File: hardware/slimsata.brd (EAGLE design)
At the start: 100 x 80 mm, 2 parts

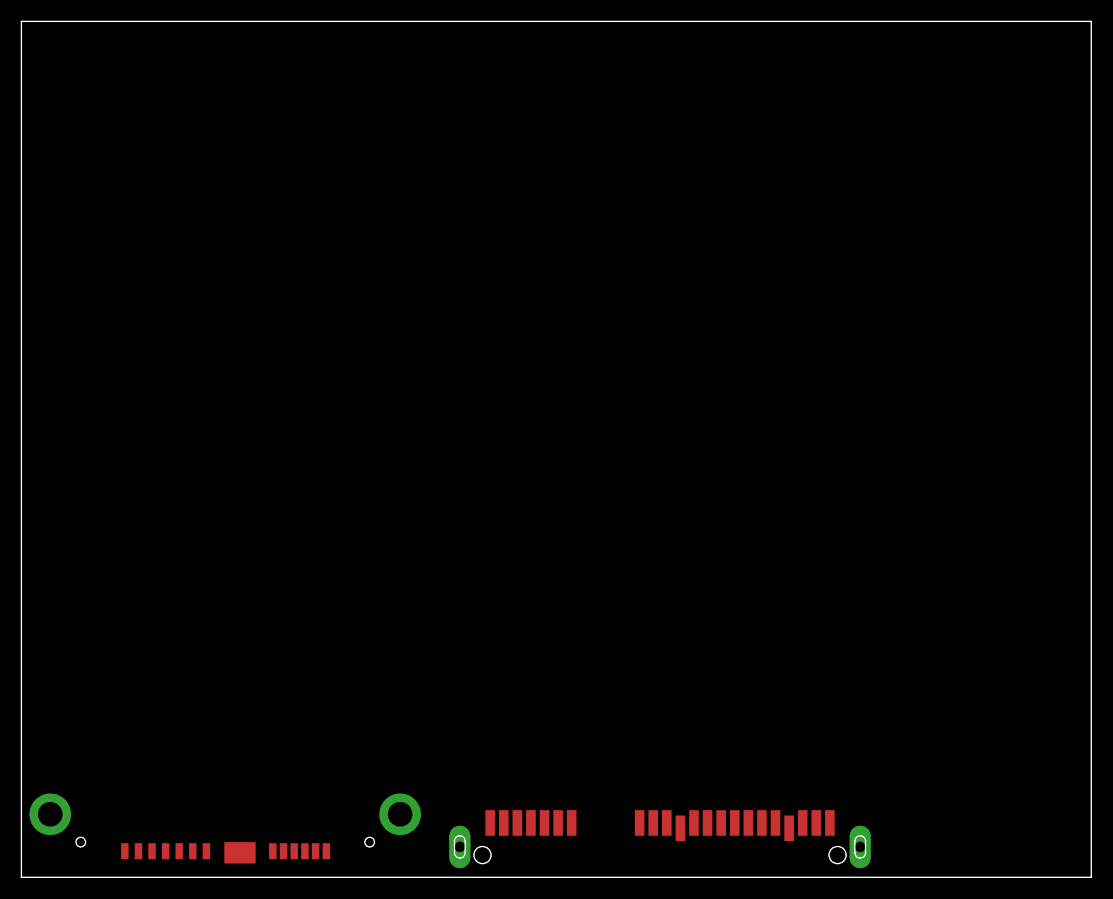
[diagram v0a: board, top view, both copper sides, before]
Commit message: Stecker neu platziert
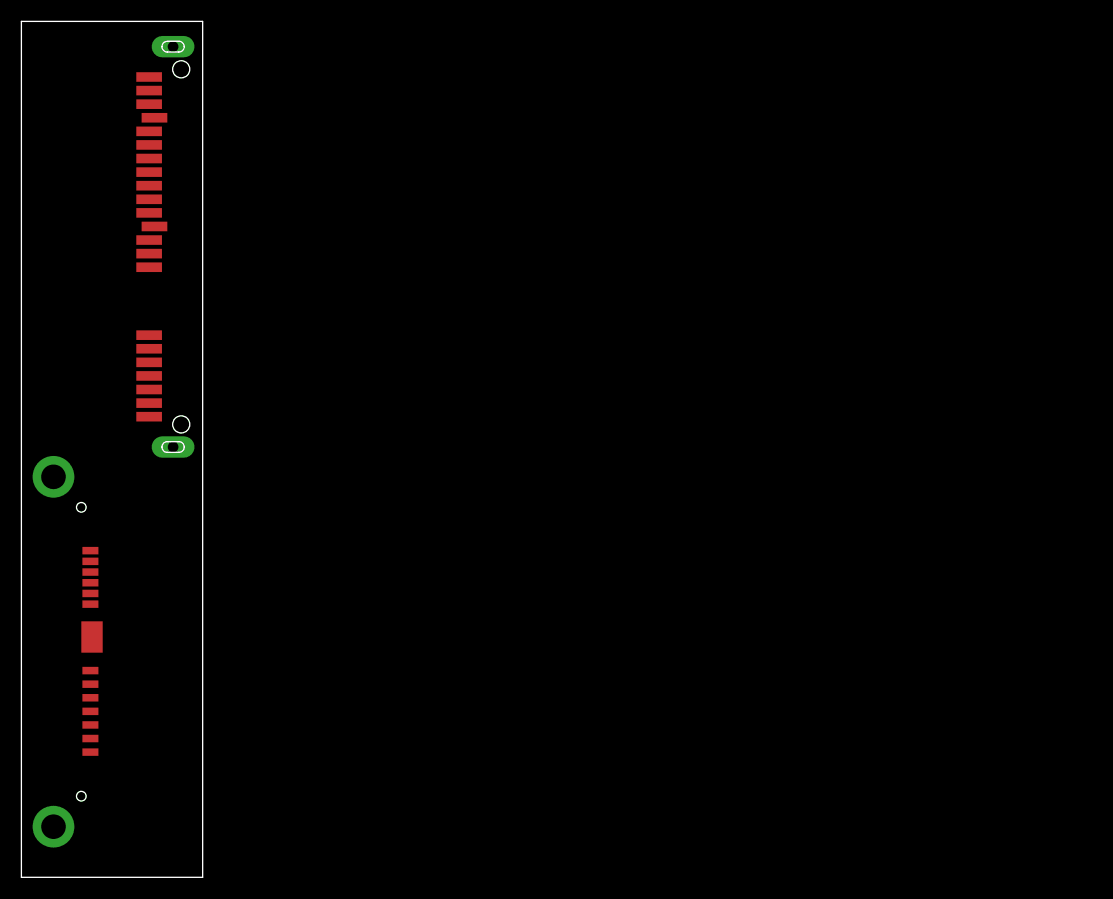
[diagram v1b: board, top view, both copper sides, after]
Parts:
- moved CON1 72.8 mm to (17.0, 58.9), turned to 90 degrees
- moved CON2 22.6 mm to (0.00, 21.1), turned to 270 degrees
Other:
- board size 100 x 80 mm -> 16.9 x 80 mm
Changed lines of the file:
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@@
 <board>
 <plain>
-<wire x1="0" y1="0" x2="100" y2="0" width="0" layer="20"/>
-<wire x1="100" y1="0" x2="100" y2="80" width="0" layer="20"/>
-<wire x1="100" y1="80" x2="0" y2="80" width="0" layer="20"/>
+<wire x1="0" y1="0" x2="16.942" y2="0" width="0" layer="20"/>
+<wire x1="16.942" y1="0" x2="16.942" y2="80" width="0" layer="20"/>
+<wire x1="16.942" y1="80" x2="0" y2="80" width="0" layer="20"/>
 <wire x1="0" y1="80" x2="0" y2="0" width="0" layer="20"/>
 </plain>
@@
 </autorouter>
 <elements>
-<element name="CON1" library="sata" package="MOLEX_47018" value="" x="59.69" y="0"/>
-<element name="CON2" library="sata" package="MOLEX_47300-1005" value="" x="19.05" y="8.89" rot="R180"/>
+<element name="CON1" library="sata" package="MOLEX_47018" value="" x="17.018" y="58.928" rot="R90"/>
+<element name="CON2" library="sata" package="MOLEX_47300-1005" value="" x="0" y="21.082" rot="R270"/>
 </elements>
 <signals>
@@
 <contactref element="CON2" pad="P6"/>
 <contactref element="CON2" pad="P5"/>
-<wire x1="35.4" y1="5.89" x2="40.98" y2="2.84" width="0" layer="19" extent="1-1"/>
-<wire x1="28.5" y1="2.44" x2="35.4" y2="5.89" width="0" layer="19" extent="1-1"/>
-<wire x1="27.5" y1="2.44" x2="28.5" y2="2.44" width="0" layer="19" extent="1-1"/>
-<wire x1="20.43" y1="2.29" x2="27.5" y2="2.44" width="0" layer="19" extent="1-1"/>
-<wire x1="62.865" y1="5.08" x2="20.43" y2="2.29" width="0" layer="19" extent="1-1"/>
-<wire x1="64.135" y1="5.08" x2="62.865" y2="5.08" width="0" layer="19" extent="1-1"/>
-<wire x1="61.595" y1="4.58" x2="62.865" y2="5.08" width="0" layer="19" extent="1-1"/>
-<wire x1="69.215" y1="5.08" x2="64.135" y2="5.08" width="0" layer="19" extent="1-1"/>
-<wire x1="71.755" y1="4.58" x2="69.215" y2="5.08" width="0" layer="19" extent="1-1"/>
-<wire x1="78.4" y1="2.84" x2="71.755" y2="4.58" width="0" layer="19" extent="1-1"/>
-<wire x1="2.7" y1="5.89" x2="78.4" y2="2.84" width="0" layer="19" extent="1-1"/>
+<wire x1="12.438" y1="70.993" x2="14.178" y2="77.638" width="0" layer="19" extent="1-1"/>
+<wire x1="11.938" y1="68.453" x2="12.438" y2="70.993" width="0" layer="19" extent="1-1"/>
+<wire x1="11.938" y1="63.373" x2="11.938" y2="68.453" width="0" layer="19" extent="1-1"/>
+<wire x1="11.938" y1="62.103" x2="11.938" y2="63.373" width="0" layer="19" extent="1-1"/>
+<wire x1="12.438" y1="60.833" x2="11.938" y2="62.103" width="0" layer="19" extent="1-1"/>
+<wire x1="14.178" y1="40.218" x2="12.438" y2="60.833" width="0" layer="19" extent="1-1"/>
+<wire x1="3" y1="37.432" x2="14.178" y2="40.218" width="0" layer="19" extent="1-1"/>
+<wire x1="6.45" y1="30.532" x2="3" y2="37.432" width="0" layer="19" extent="1-1"/>
+<wire x1="6.45" y1="29.532" x2="6.45" y2="30.532" width="0" layer="19" extent="1-1"/>
+<wire x1="6.6" y1="22.462" x2="6.45" y2="29.532" width="0" layer="19" extent="1-1"/>
+<wire x1="3" y1="4.732" x2="6.6" y2="22.462" width="0" layer="19" extent="1-1"/>
 </signal>
 <signal name="N$2">
@@
 <contactref element="CON1" pad="S7"/>
 <contactref element="CON2" pad="S7"/>
-<wire x1="47.625" y1="5.08" x2="43.815" y2="5.08" width="0" layer="19" extent="1-1"/>
-<wire x1="51.435" y1="5.08" x2="47.625" y2="5.08" width="0" layer="19" extent="1-1"/>
-<wire x1="17.29" y1="2.44" x2="51.435" y2="5.08" width="0" layer="19" extent="1-1"/>
-<wire x1="13.48" y1="2.44" x2="17.29" y2="2.44" width="0" layer="19" extent="1-1"/>
-<wire x1="9.67" y1="2.44" x2="13.48" y2="2.44" width="0" layer="19" extent="1-1"/>
+<wire x1="11.938" y1="46.863" x2="11.938" y2="50.673" width="0" layer="19" extent="1-1"/>
+<wire x1="11.938" y1="43.053" x2="11.938" y2="46.863" width="0" layer="19" extent="1-1"/>
+<wire x1="6.45" y1="19.322" x2="11.938" y2="43.053" width="0" layer="19" extent="1-1"/>
+<wire x1="6.45" y1="15.512" x2="6.45" y2="19.322" width="0" layer="19" extent="1-1"/>
+<wire x1="6.45" y1="11.702" x2="6.45" y2="15.512" width="0" layer="19" extent="1-1"/>
 </signal>
 <signal name="N$5">
 <contactref element="CON1" pad="S2"/>
 <contactref element="CON2" pad="S2"/>
-<wire x1="10.94" y1="2.44" x2="45.085" y2="5.08" width="0" layer="19" extent="1-1"/>
+<wire x1="6.45" y1="12.972" x2="11.938" y2="44.323" width="0" layer="19" extent="1-1"/>
 </signal>
 <signal name="N$6">
 <contactref element="CON1" pad="S3"/>
 <contactref element="CON2" pad="S3"/>
-<wire x1="12.21" y1="2.44" x2="46.355" y2="5.08" width="0" layer="19" extent="1-1"/>
+<wire x1="6.45" y1="14.242" x2="11.938" y2="45.593" width="0" layer="19" extent="1-1"/>
 </signal>
 <signal name="N$7">
 <contactref element="CON1" pad="S5"/>
 <contactref element="CON2" pad="S5"/>
-<wire x1="14.75" y1="2.44" x2="48.895" y2="5.08" width="0" layer="19" extent="1-1"/>
+<wire x1="6.45" y1="16.782" x2="11.938" y2="48.133" width="0" layer="19" extent="1-1"/>
 </signal>
 <signal name="N$8">
 <contactref element="CON1" pad="S6"/>
 <contactref element="CON2" pad="S6"/>
-<wire x1="16.02" y1="2.44" x2="50.165" y2="5.08" width="0" layer="19" extent="1-1"/>
+<wire x1="6.45" y1="18.052" x2="11.938" y2="49.403" width="0" layer="19" extent="1-1"/>
 </signal>
 <signal name="N$3">
@@
 <contactref element="CON2" pad="P2"/>
 <contactref element="CON2" pad="P3"/>
-<wire x1="66.675" y1="5.08" x2="65.405" y2="5.08" width="0" layer="19" extent="1-1"/>
-<wire x1="67.945" y1="5.08" x2="66.675" y2="5.08" width="0" layer="19" extent="1-1"/>
-<wire x1="24.5" y1="2.44" x2="65.405" y2="5.08" width="0" layer="19" extent="1-1"/>
-<wire x1="25.5" y1="2.44" x2="24.5" y2="2.44" width="0" layer="19" extent="1-1"/>
+<wire x1="11.938" y1="65.913" x2="11.938" y2="67.183" width="0" layer="19" extent="1-1"/>
+<wire x1="11.938" y1="64.643" x2="11.938" y2="65.913" width="0" layer="19" extent="1-1"/>
+<wire x1="6.45" y1="27.532" x2="11.938" y2="64.643" width="0" layer="19" extent="1-1"/>
+<wire x1="6.45" y1="26.532" x2="6.45" y2="27.532" width="0" layer="19" extent="1-1"/>
 </signal>
 </signals>
